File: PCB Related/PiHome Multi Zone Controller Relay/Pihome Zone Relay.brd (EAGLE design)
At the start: 100.6 x 75.6 mm, 18 parts, among them IC1 REG1117, M1 WIRELESS-NRF24L01, M3 ARDUINO-PRO-MINI-5.0V

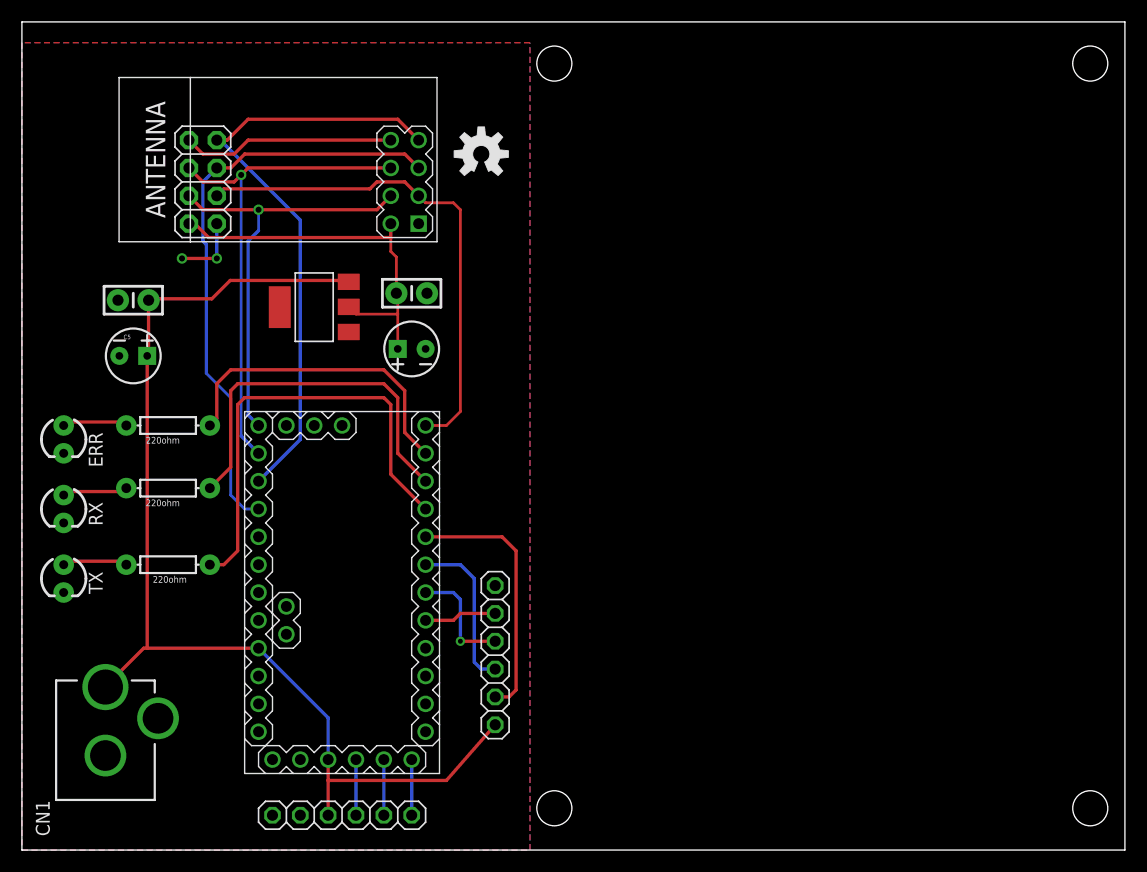
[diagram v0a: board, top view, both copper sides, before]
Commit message: Improved PCB Design
Improved PCB Design
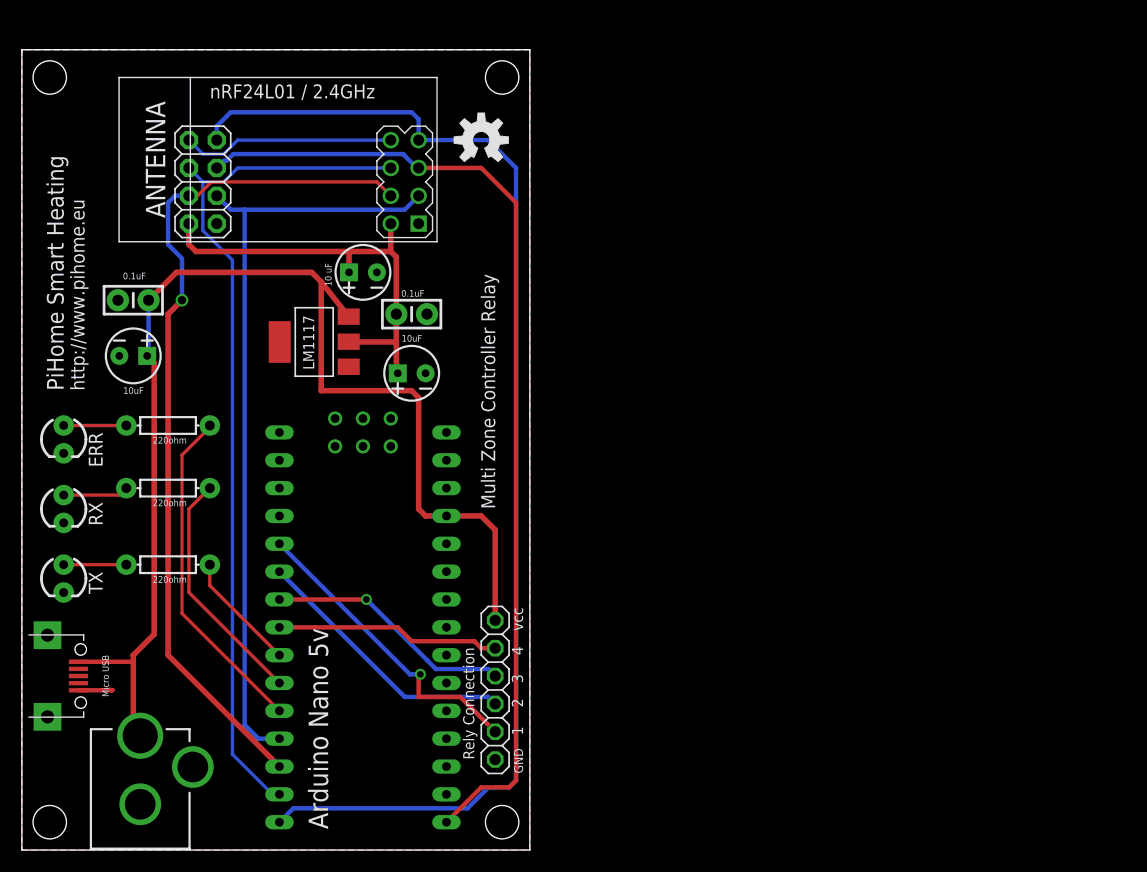
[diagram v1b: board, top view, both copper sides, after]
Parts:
- removed JP1: (no value), adafruit:1X06
- removed M3: ARDUINO-PRO-MINI-5.0V, diy-modules:ARDUINO-PRO-MINI
- added C1: 10uf, SparkFun-Capacitors:CPOL-RADIAL-10UF-25V-KIT
- added U$1: NANO, Arduino Pro Mini-Nano:NANO
- added U$2: MICRO-USB, microusb:MICRO-USB
- moved CN1 5.46 mm to (10.8, -3.17)
- moved IC1 3.18 mm to (26.7, 46.4)
- moved JP2 3.18 mm to (43.2, 14.6), turned to 90 degrees
- moved C6 2.22 mm to (35.6, 43.5)
- moved C4 1.90 mm to (35.6, 48.9)
- moved LOGO4 1.27 mm to (41.9, 64.8)
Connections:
- removed net DTR: JP1.1, M3.J1.6
- removed net IN01: JP2.2, M3.J7.8
- removed net IN02: JP2.3, M3.J7.7
- removed net IN03: JP2.4, M3.J7.6
- removed net IN04: JP2.5, M3.J7.5
- removed net RAW: M3.J6.1
- removed net RXD: JP1.3, M3.J1.4
- removed net TXD: JP1.2, M3.J1.5
- new net ZONE_01: JP2.2, U$1.D2
- new net ZONE_02: JP2.3, U$1.D3
- new net ZONE_03: JP2.4, U$1.D4
- new net ZONE_04: JP2.5, U$1.D5
- net CE: now also U$1.D9; no longer M3.J7.1
- net CSN: now also U$1.D10; no longer M3.J6.12
- net ERR_LED: now also U$1.D8; no longer M3.J7.2
- net GND: now also C1.2, U$1.GND, U$1.GND1, U$2.5, U$2.GND1, U$2.GND2; no longer JP1.5, JP1.6, M3.J1.1, M3.J1.2, M3.J6.2, M3.J7.9
- net MISO: now also U$1.D12; no longer M3.J6.10
- net MOSI: now also U$1.D11; no longer M3.J6.11
- net RX_LED: now also U$1.D7; no longer M3.J7.3
- net SCK: now also U$1.D13; no longer M3.J6.9
- net TX_LED: now also U$1.D6; no longer M3.J7.4
- net VCC_3.3: now also C1.1
- net VCC_5: now also U$1.5V, U$2.1; no longer JP1.4, M3.J1.3, M3.J6.4
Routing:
- net MISO: track 56.0 -> 111.5 mm
- net CSN: track 39.9 -> 81.9 mm
- net SCK: track 54.0 -> 90.3 mm
- net MOSI: track 45.5 -> 78.6 mm, vias 1 -> 0
- net TX_LED: track 41.7 -> 10.9 mm
- net ZONE_01: track 0.00 -> 28.2 mm, vias 0 -> 1
- net ZONE_02: track 0.00 -> 24.7 mm
- net CE: track 46.3 -> 70.8 mm
- net IN04: track 23.6 -> 0.00 mm
- net ZONE_03: track 0.00 -> 22.6 mm, vias 0 -> 1
- net ZONE_04: track 0.00 -> 20.5 mm
- net IN03: track 14.8 -> 0.00 mm
- net RX_LED: track 34.4 -> 22.0 mm
- net VCC_5: track 101.7 -> 112.8 mm
- net IN02: track 10.6 -> 0.00 mm, vias 1 -> 0
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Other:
- board size 100.6 x 75.6 mm -> 46.3 x 73 mm
- board text added: "0.1uF"
- board text added: "1"
- board text added: "10 uF"
- board text added: "10uF"
- board text added: "2"
- board text added: "3"
- board text added: "4"
- board text added: "Arduino Nano 5v"
- board text added: "LM1117"
- board text added: "Micro USB"
- board text added: "Multi Zone Controller Relay"
- board text added: "PiHome Smart Heating"
- board text added: "Rely Connection"
- board text added: "http://www.pihome.eu"
- board text added: "nRF24L01 / 2.4GHz"
- board text removed: "4 Channel SainSmart Relay Board"
- board text removed: "DTR"
- board text removed: "RXD"
- board text removed: "TXD"
